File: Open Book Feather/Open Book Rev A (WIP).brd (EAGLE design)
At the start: 77.5 x 112.3 mm, 115 parts, among them J1 SJ-43514-SMT, J2 10118193-0001LF, Q1 DMG341, Q2 IRLML0100, SW1 SPDT_SWITCH, U1 AP2112-3.3, U2 MCP73831T-2ACI/OT, U3 ATSAMD51J64-TQFP(10X10), U4 GD25Q16C (or GD25Q32C), U5 74AC165D, U6 GD25Q16C (or GD25Q32C), U7 23K256-I/SN, X1 JSTPH, X2 2x5 0.05" SWD

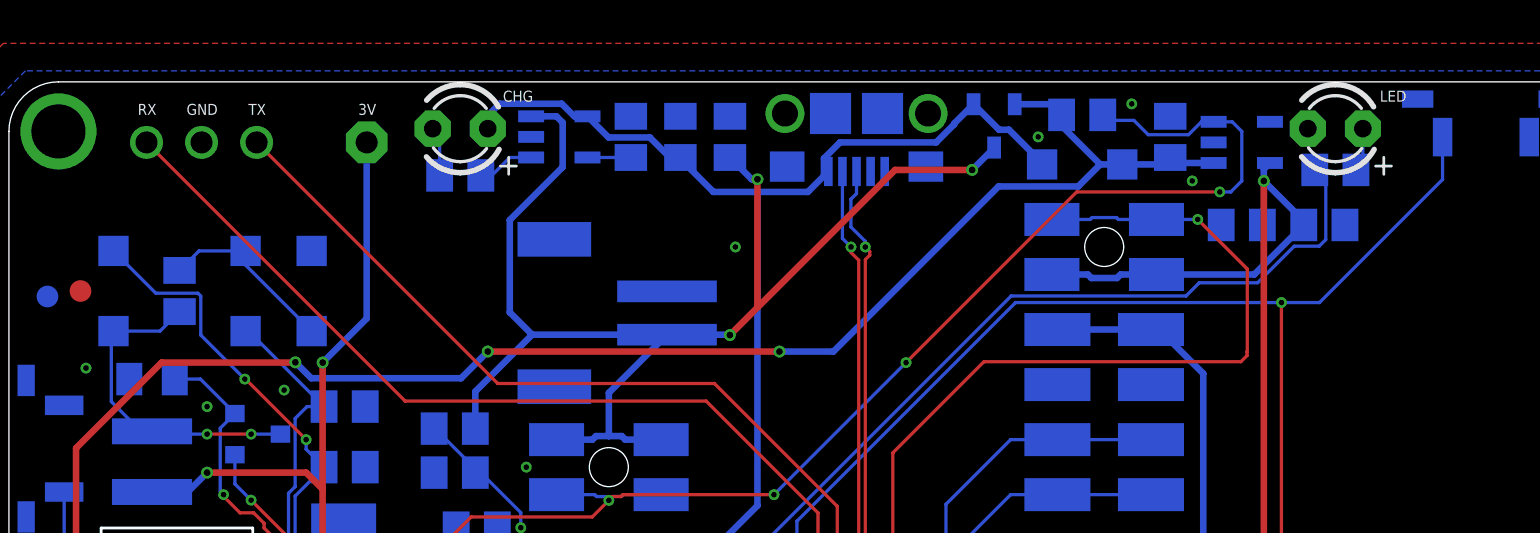
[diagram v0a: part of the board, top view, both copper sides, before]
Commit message: add these cool right-angle LEDs (that i ordered too many of)
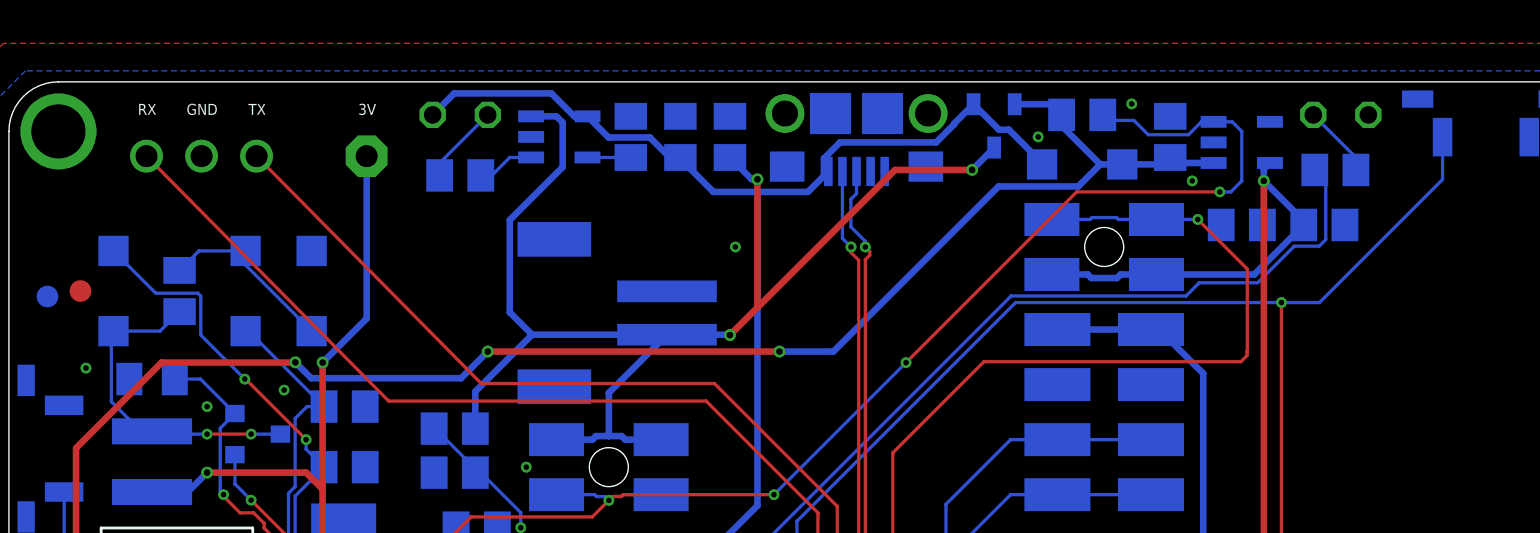
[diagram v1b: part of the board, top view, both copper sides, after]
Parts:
- CHG, LED: device adafruit:LED3MM -> adafruit:LED17X45_SIDEVIEW
- moved LED 0.68 mm to (61.2, 110.7), flipped to the bottom
- moved CHG 0.64 mm to (20.6, 110.7), flipped to the bottom
- moved JP1 0.64 mm to (8.64, 108.8)
- moved JP2 0.64 mm to (16.3, 108.8)
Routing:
- net VBUS: track 56.1 -> 58.4 mm
- net N$4: track 2.29 -> 3.71 mm
- net N$7: track 2.04 -> 3.35 mm
- net +3V3: track 449.6 -> 448.9 mm
